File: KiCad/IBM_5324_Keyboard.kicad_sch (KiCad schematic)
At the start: 96 parts, among them J1 To 5324, J2 To DB25, SW1 CMD, SW10 ERASE, SW11 | 1, SW12 # 3, SW13 % 5, SW14 & 7, SW15 * +, SW16 ( 9, SW17 _ -, SW18 RH <-, SW19 / -, SW2 ~ `, SW20 NP 8, SW21 HOLD, SW22 FIELD ADV, SW23 W, SW24 R, SW25 Y, SW26 I, SW27 P, SW28 | \, SW29 NP 7, SW3 @ 2, SW30 NP 9, SW31 INQ, SW32 SHIFT LOCK, SW33 Q, SW34 E, SW35 T, SW36 O, SW37 ! ¢, SW38 ENTER, SW39 NP 4, SW4 $ 4, SW40 FIELD-, SW41 U, SW42 ERROR RESET, SW43 LH SHIFT, SW44 A, SW45 D, SW46 G, SW47 J, SW48 L, SW49 " ', SW5 ^ 6, SW50 } {, SW51 NP 5, SW52 NP 6, SW53 TEST, SW54 SCROLL DOWN, SW55 S, SW56 F, SW57 H, SW58 SCROLL UP, SW59 K, SW6 * 8, SW60 : ;, SW61 NEWLINE, SW62 NP 1, SW63 NP 3, SW64 ->, SW65 > <, SW66 C, SW67 B, SW68 M, SW69 . ., SW7 ) 0, SW70 RH SHIFT, SW71 NP 2, SW72 FIELD+, SW73 N, SW74 LH <-, SW75 ALT, SW76 Z, SW77 X, SW78 V, SW79 SPACE, SW8 + =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

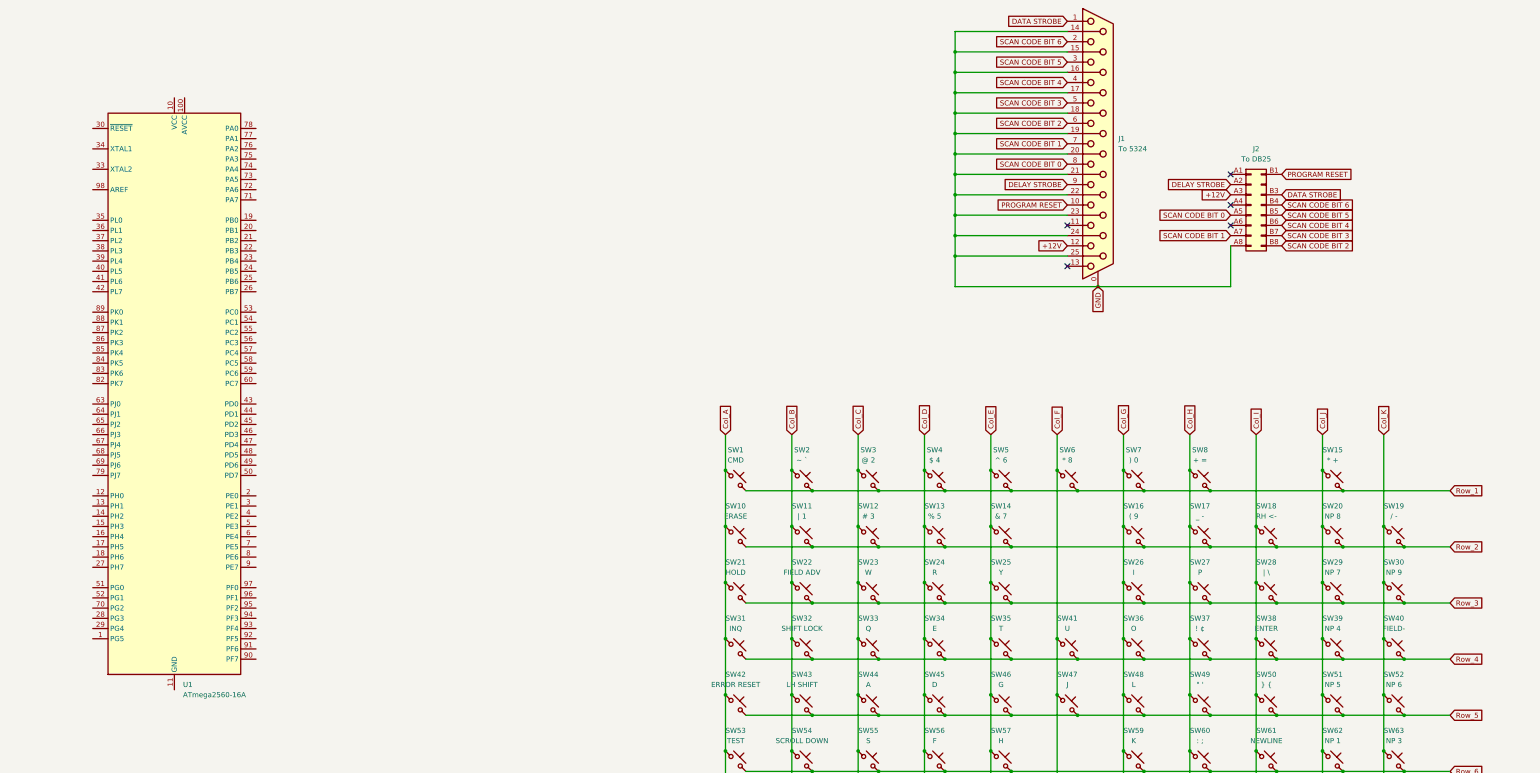
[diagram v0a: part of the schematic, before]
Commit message: Started firmware development
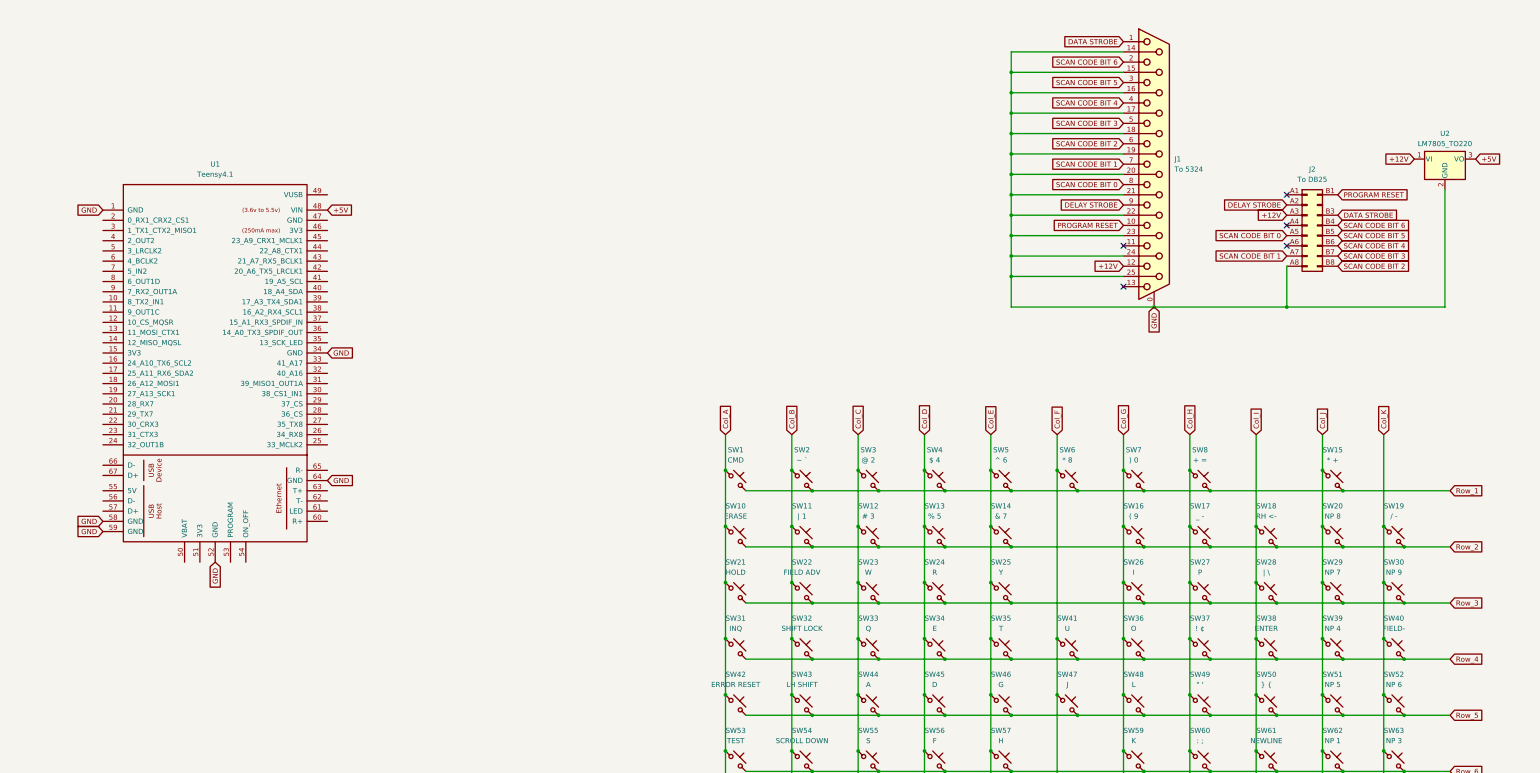
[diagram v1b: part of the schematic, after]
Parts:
- removed U1: ATmega2560-16A, Package_QFP:TQFP-100_14x14mm_P0.5mm, symbol MCU_Microchip_ATmega:ATmega2560-16A
- added U1: Teensy4.1, Clueless_Engineer:Teensy41, symbol teensy:Teensy4.1
- added U2: LM7805_TO220, Package_TO_SOT_THT:TO-220-3_Horizontal_TabDown, symbol Regulator_Linear:LM7805_TO220
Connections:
- net +12V: now also U2.1 (VI)
- net GND: now also U1.1 (GND), U1.34 (GND), U1.52 (GND), U1.58 (GND), U1.59 (GND), U1.64 (GND), U2.2 (GND)
- new net +5V: U1.48 (VIN), U2.3 (VO)
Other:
- moved on the sheet: J1, J2
